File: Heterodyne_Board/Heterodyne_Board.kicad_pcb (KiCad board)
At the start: 2 copper layers, 70.4 x 69.4 mm, 63 parts, among them J1 Barrel_Jack, J2 SWITCH, J3 LED, J4 AudioJack2_Ground_Switch, J5 Speaker, J6 Microphone, J7 AVR-ISP-6, J8 AVR-ISP-6, SW1 SW_SPST, SW2 SW_SPST, U1 AP2112K-3.3, U2 LM386, U3 TLV9054xD, U4 ATtiny85-20P, U5 TS5A3159DCK, U6 W25X40CLSN

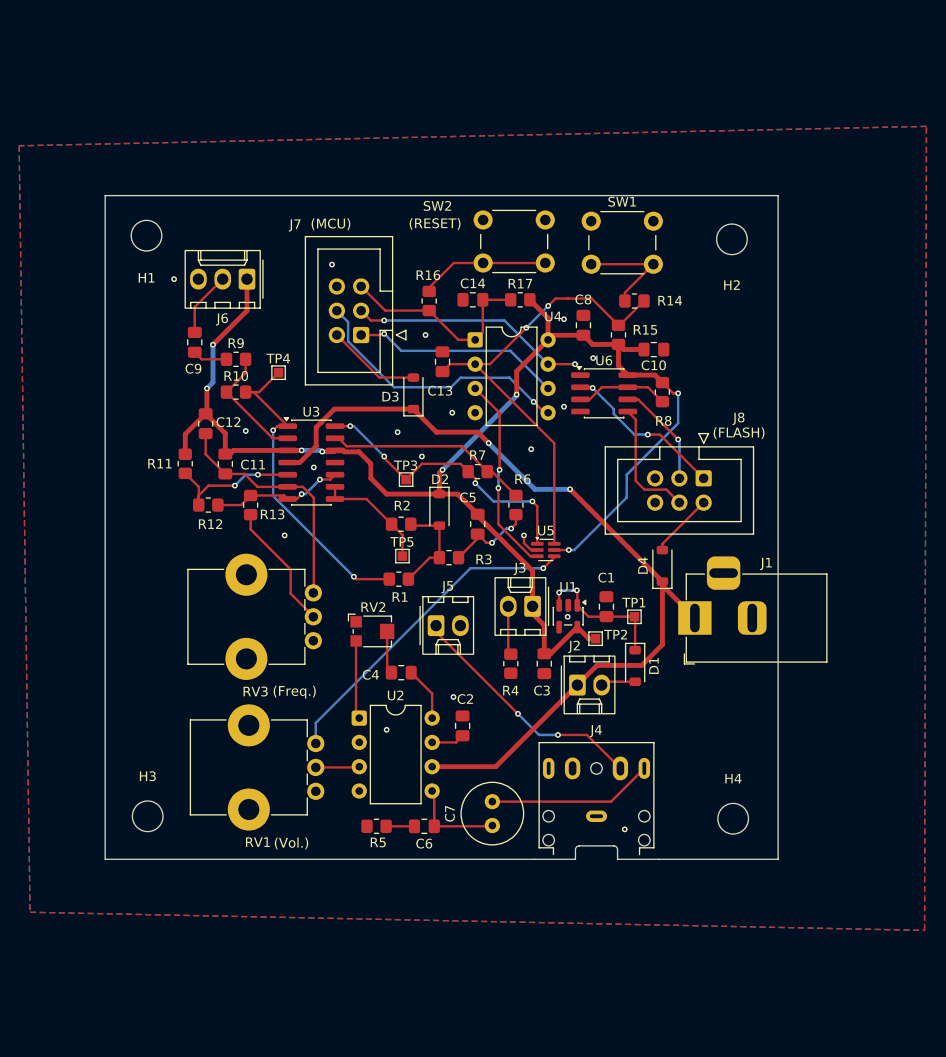
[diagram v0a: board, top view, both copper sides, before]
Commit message: FINAL BOARD REV
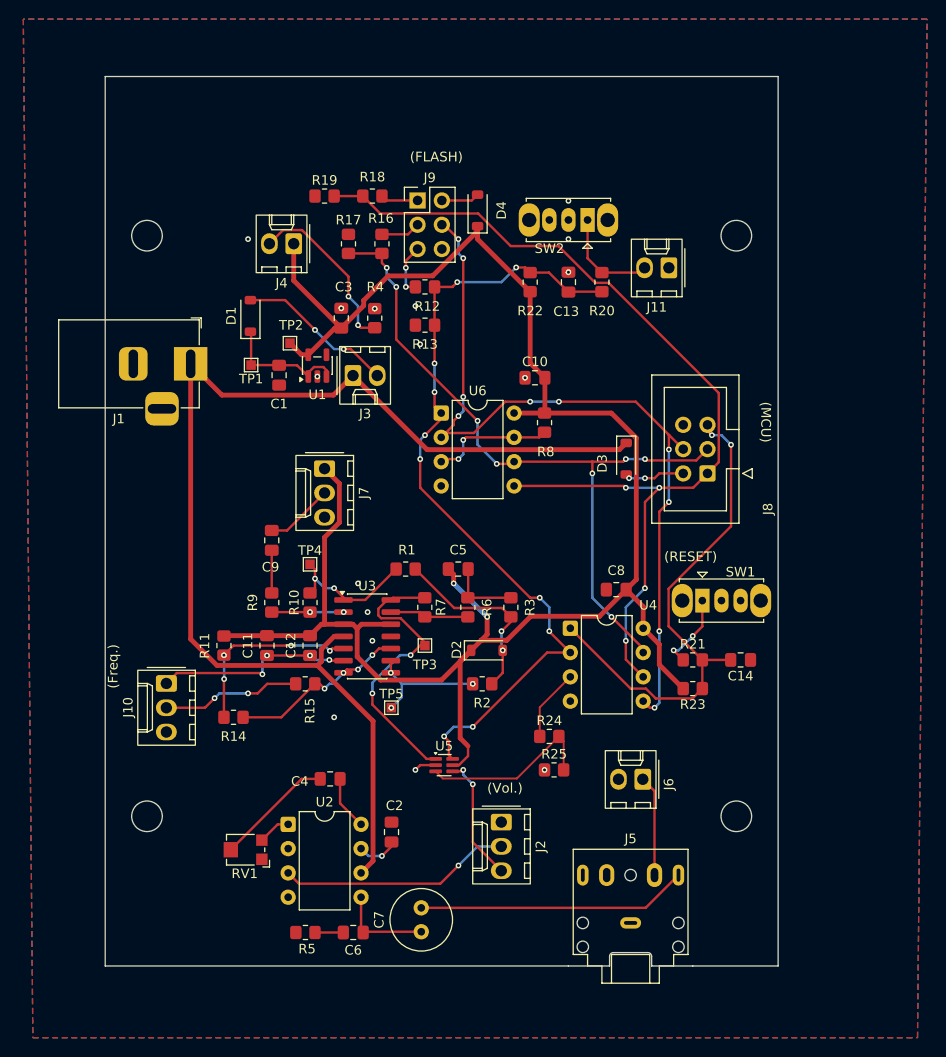
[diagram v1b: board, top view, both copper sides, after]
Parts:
- removed RV2: R_Potentiometer_Trim, Potentiometer_SMD:Potentiometer_Bourns_TC33X_Vertical
- removed RV3: R_Potentiometer, Potentiometer_THT:Potentiometer_Bourns_PTV09A-1_Single_Vertical
- added J10: Frequenciometer, Connector_Molex:Molex_KK-254_AE-6410-03A_1x03_P2.54mm_Vertical, F.Cu at (145.5, 111.5)
- added J11: Audio_EN, Connector_Molex:Molex_KK-254_AE-6410-02A_1x02_P2.54mm_Vertical, F.Cu at (198.0, 68.0)
- added J9: AVR-ISP-6, Connector_PinHeader_2.54mm:PinHeader_2x03_P2.54mm_Vertical, F.Cu at (171.7, 61.0)
- added R18: 470, Resistor_SMD:R_0805_2012Metric_Pad1.20x1.40mm_HandSolder, F.Cu at (167.0, 60.5)
- added R19: 1k, Resistor_SMD:R_0805_2012Metric_Pad1.20x1.40mm_HandSolder, F.Cu at (162.0, 60.5)
- added R20: 1k, Resistor_SMD:R_0805_2012Metric_Pad1.20x1.40mm_HandSolder, F.Cu at (191.0, 69.5)
- added R21: 1k, Resistor_SMD:R_0805_2012Metric_Pad1.20x1.40mm_HandSolder, F.Cu at (200.5, 109.0)
- added R22: 10k, Resistor_SMD:R_0805_2012Metric_Pad1.20x1.40mm_HandSolder, F.Cu at (183.5, 69.5)
- added R23: 10k, Resistor_SMD:R_0805_2012Metric_Pad1.20x1.40mm_HandSolder, F.Cu at (200.5, 112.0)
- added R24: 10k, Resistor_SMD:R_0805_2012Metric_Pad1.20x1.40mm_HandSolder, F.Cu at (185.5, 117.0)
- added R25: 1k, Resistor_SMD:R_0805_2012Metric_Pad1.20x1.40mm_HandSolder, F.Cu at (186.0, 120.5)
- J2: value SWITCH -> Volume; footprint Connector_Molex:Molex_KK-254_AE-6410-02A_1x02_P2.54mm_Vertical -> Connector_Molex:Molex_KK-254_AE-6410-03A_1x03_P2.54mm_Vertical
- J3: value LED -> SWITCH
- J4: value AudioJack2_Ground_Switch -> LED; footprint Connector_Audio:Jack_3.5mm_CUI_SJ1-3525N_Horizontal -> Connector_Molex:Molex_KK-254_AE-6410-02A_1x02_P2.54mm_Vertical
- J5: value Speaker -> AudioJack2_Ground_Switch; footprint Connector_Molex:Molex_KK-254_AE-6410-02A_1x02_P2.54mm_Vertical -> Connector_Audio:Jack_3.5mm_CUI_SJ1-3525N_Horizontal
- J6: value Microphone -> Speaker; footprint Connector_Molex:Molex_KK-254_AE-6410-03A_1x03_P2.54mm_Vertical -> Connector_Molex:Molex_KK-254_AE-6410-02A_1x02_P2.54mm_Vertical
- J7: value AVR-ISP-6 -> Microphone; footprint Connector_IDC:IDC-Header_2x03_P2.54mm_Vertical -> Connector_Molex:Molex_KK-254_AE-6410-03A_1x03_P2.54mm_Vertical
- R12, R16: value 1k -> 470
- R13: value 100 -> 1k
- R15: value 10k -> 100
- R17: value 10k -> 1k
- RV1: value R_Potentiometer -> R_Potentiometer_Trim; footprint Potentiometer_THT:Potentiometer_Bourns_PTV09A-1_Single_Vertical -> Potentiometer_SMD:Potentiometer_Bourns_TC33X_Vertical
- SW1, SW2: value SW_SPST -> SW_SPDT; footprint Button_Switch_THT:SW_PUSH_6mm_H5mm -> Button_Switch_THT:SW_Slide_SPDT_Straight_CK_OS102011MS2Q
- U6: value W25X40CLSN -> SST25VF080B; footprint Package_SO:SOIC-8_3.9x4.9mm_P1.27mm -> Package_DIP:DIP-8_W7.62mm
- moved J4 67.7 mm to (158.8, 65.5), turned to 180 degrees
- moved J6 66.7 mm to (195.3, 121.5)
- moved R14 60.4 mm to (152.5, 115.0)
- moved J1 59.0 mm to (148.0, 78.0), turned to 0 degrees
- moved D1 54.4 mm to (154.2, 73.0), turned to 90 degrees
- moved R15 49.0 mm to (160.0, 111.5), turned to 180 degrees
- moved TP1 48.0 mm to (154.3, 78.2), turned to 180 degrees
- moved C14 46.9 mm to (205.5, 109.0), turned to 180 degrees
- moved TP2 44.4 mm to (158.4, 75.9), turned to 180 degrees
- moved C1 41.9 mm to (157.2, 79.2), turned to -90 degrees
- moved C3 41.9 mm to (163.7, 73.3), turned to 90 degrees
- moved D4 41.9 mm to (178.0, 62.0)
- moved SW1 41.3 mm to (201.5, 102.8)
- moved R4 38.8 mm to (167.2, 73.3), turned to 90 degrees
- moved J5 37.1 mm to (194.0, 136.5)
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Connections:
- C13 pad 2: /Audio_EN -> /CANS
- C14 pad 2: /RESET_MCU -> /RESET
- C9 pad 1: Net-(J6-Pin_2) -> Net-(J7-Pin_2)
- D4 pad 1: +6V -> +3V3
- J2 pad 1: +6V -> GND
- J2 pad 2: Net-(D1-A) -> Net-(J2-Pin_2)
- J3 pad 1: +3V3 -> +6V
- J3 pad 2: Net-(J3-Pin_2) -> Net-(D1-A)
- J6 pad 1: +3V3 -> Net-(J6-Pin_1)
- J6 pad 2: Net-(J6-Pin_2) -> GND
- J7 pad 1: /MISO_MCU -> +3V3
- J7 pad 2: Net-(D3-A) -> Net-(J7-Pin_2)
- J7 pad 3: /SCK_MCU -> GND
- J8 pad 1: /MISO_FLASH -> /MISO
- J8 pad 2: Net-(D4-A) -> Net-(D3-A)
- J8 pad 3: /SCK_FLASH -> /SCK
- J8 pad 4: /MOSI_FLASH -> /MOSI
- J8 pad 5: unconnected-(J8-~{RST}-Pad5) -> /RESET
- R12 pad 1: Net-(U3B-+) -> Net-(J9-~{RST})
- R12 pad 2: Net-(U3C-+) -> /CANS
- R13 pad 1: Net-(U3C-+) -> GND
- R13 pad 2: Net-(R13-Pad2) -> /CANS
- R14 pad 1: Net-(SW1-B) -> Net-(U3B-+)
- R14 pad 2: /Audio_EN -> Net-(U3C-+)
- R15 pad 1: /Audio_EN -> Net-(U3C-+)
- R15 pad 2: +3V3 -> Net-(J10-Pin_2)
- R16 pad 1: Net-(SW2-B) -> Net-(J9-SCK)
- R16 pad 2: /RESET_MCU -> /SCK
- R17 pad 1: /RESET_MCU -> GND
- R17 pad 2: +3V3 -> /SCK
- R4 pad 1: Net-(J3-Pin_2) -> Net-(J4-Pin_2)
- RV1 pad 1: /Speaker_in -> unconnected-(RV1-Pad1)
- RV1 pad 2: Net-(U2-+) -> Net-(C4-Pad2)
- RV1 pad 3: GND -> Net-(RV1-Pad3)
- SW1 pad 1: GND -> Net-(SW1-A)
- SW1 pad 2: Net-(SW1-B) -> GND
- SW2 pad 1: GND -> Net-(J11-Pin_2)
- SW2 pad 2: Net-(SW2-B) -> GND
- U2 pad 1: Net-(RV2-Pad3) -> Net-(RV1-Pad3)
- U2 pad 3: Net-(U2-+) -> Net-(J2-Pin_2)
- U4 pad 1: /RESET_MCU -> /RESET
- U4 pad 2: /Audio_EN -> /CANS
- U4 pad 5: /MOSI_MCU -> /MOSI
- U4 pad 6: /MISO_MCU -> /MISO
- U4 pad 7: /SCK_MCU -> /SCK
- U5 pad 3: /MCU_out -> Net-(R24-Pad2)
- U5 pad 6: /Audio_EN -> /CANS
- U6 pad 1: GND -> /CANS
- U6 pad 2: /MISO_FLASH -> /MOSI
- U6 pad 5: /MOSI_FLASH -> /MISO
- U6 pad 6: /SCK_FLASH -> /SCK
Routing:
- net /MISO: track 0.00 -> 100.5 mm, vias 0 -> 4
- net /CANS: track 0.00 -> 85.5 mm, vias 0 -> 10
- net /MOSI: track 0.00 -> 83.8 mm, vias 0 -> 10
- net /SCK: track 0.00 -> 75.4 mm, vias 0 -> 8
- net /RESET: track 0.00 -> 53.6 mm, vias 0 -> 2
- net /Audio_EN: track 48.6 -> 0.00 mm, vias 2 -> 0
- net +3V3: track 150.1 -> 197.8 mm, vias 8 -> 2
- net +6V: track 91.3 -> 123.8 mm, vias 2 -> 0
- net /MOSI_MCU: track 28.5 -> 0.00 mm, vias 1 -> 0
- net Net-(J5-Pin_1): track 25.8 -> 0.00 mm, vias 2 -> 0
- net /SCK_MCU: track 24.9 -> 0.00 mm, vias 2 -> 0
- net Net-(J2-Pin_2): track 0.00 -> 24.4 mm, vias 0 -> 1
- net /MISO_MCU: track 22.1 -> 0.00 mm, vias 1 -> 0
- net /RESET_MCU: track 21.7 -> 0.00 mm
- net /Speaker_in: track 34.4 -> 13.4 mm, vias 1 -> 2
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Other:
- board size 70.4 x 69.4 mm -> 70.4 x 93 mm
